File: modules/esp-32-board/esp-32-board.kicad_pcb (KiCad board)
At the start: 2 copper layers, 53.4 x 68.6 mm, 39 parts, among them J1 Conn_01x14_Female, J2 Conn_01x18_Female, J3 Conn_01x06, J4 USB_B_Micro, J5 Barrel_Jack_MountingPin, J6 ESP-PROG-Program, J7 ESP-PROG-Debug, Q1 BCR129S, SW1 SW_Push, SW2 SW_Push, U1 ESP32-WROOM-32, U2 NCP1117-3.3, U3 NCP1117ST50T3G, U4 USBLC6-2SC6, U5 FT232RL

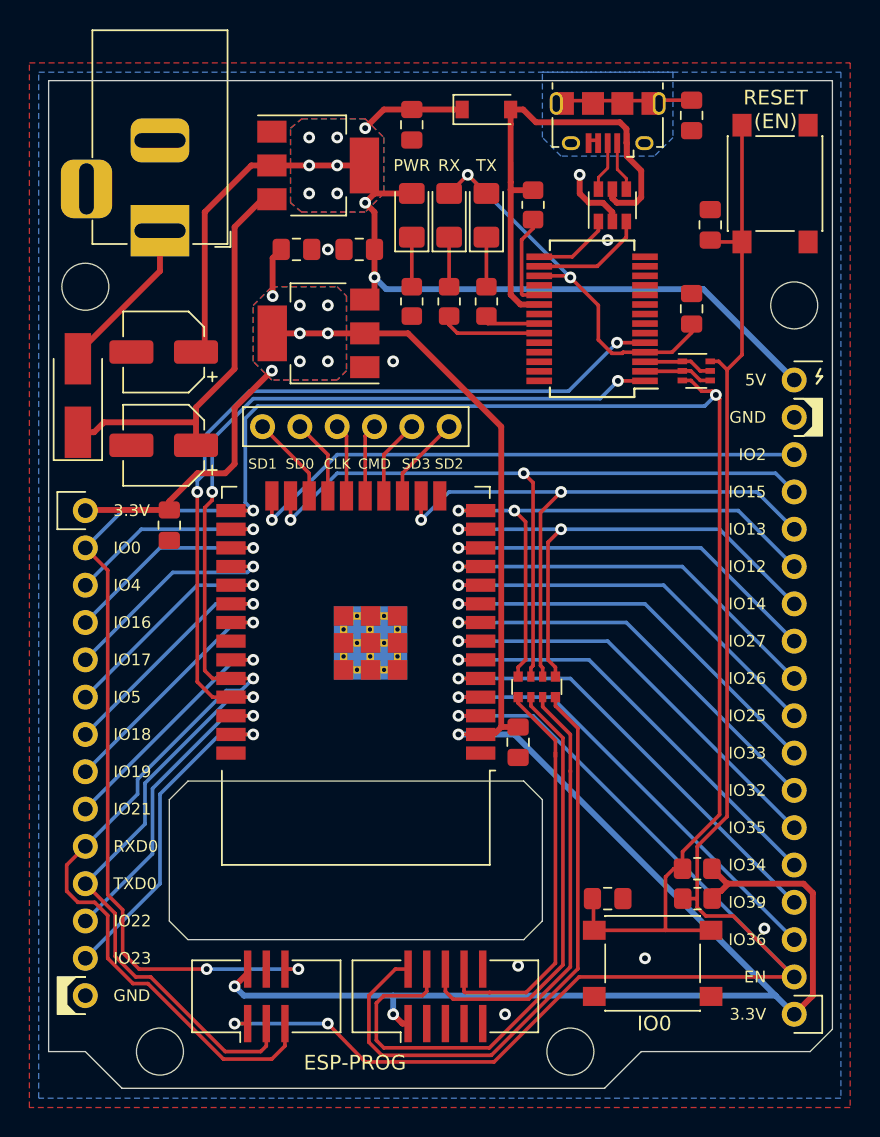
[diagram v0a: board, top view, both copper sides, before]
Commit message: Documentational changes
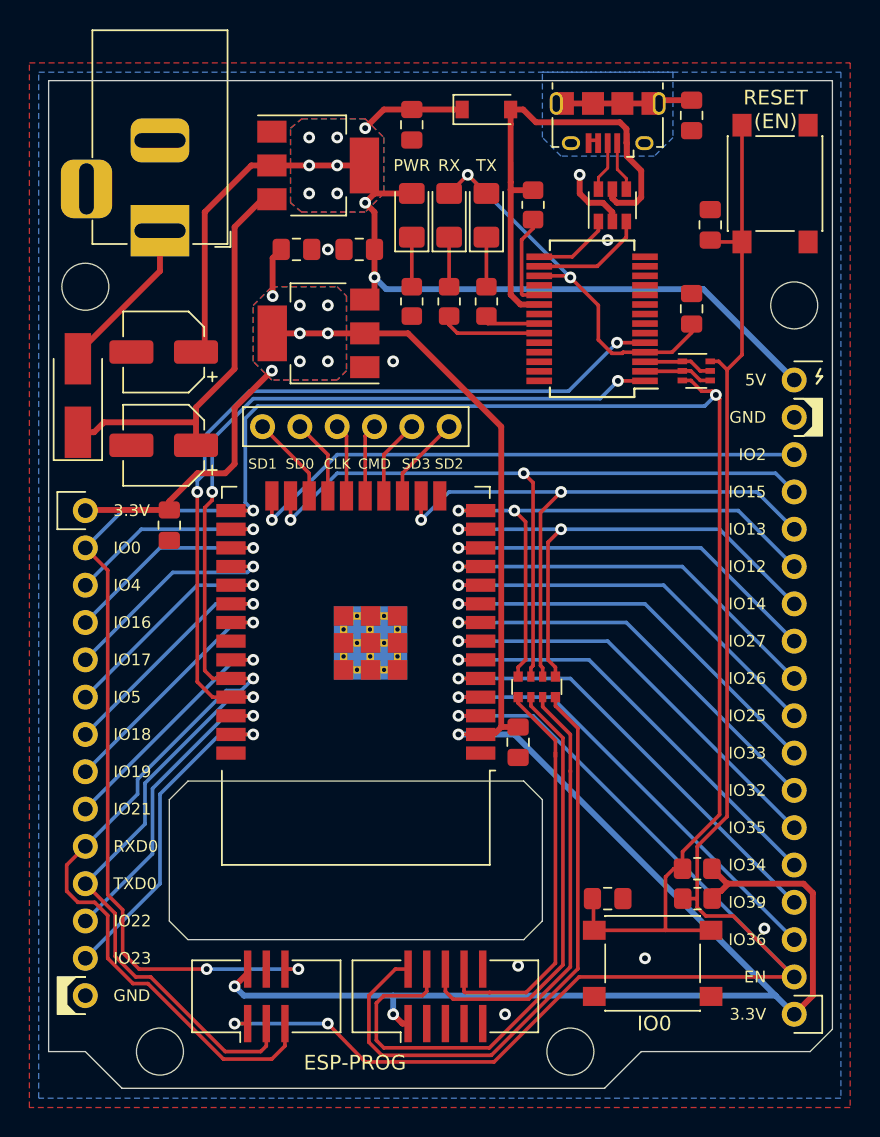
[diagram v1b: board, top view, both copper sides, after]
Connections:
- net Net-(C10-Pad1) renamed /USB/USB_SHIELD
- net Net-(D1-Pad1) renamed /Power/PWR_LED_CATHODE
- net Net-(D2-Pad2) renamed /Power/DC_INPUT
- net Net-(D4-Pad1) renamed /USB/~TXDLED'
- net Net-(D5-Pad1) renamed /USB/~RXDLED'
- net Net-(J4-Pad2) renamed /USB/USB_DN'
- net Net-(J4-Pad3) renamed /USB/USB_DP'
- net Net-(J7-Pad2) renamed /TMS'
- net Net-(J7-Pad4) renamed /TCK'
- net Net-(J7-Pad6) renamed /TDO'
- net Net-(J7-Pad8) renamed /TDI'
- net Net-(R2-Pad1) renamed /USB/USB_RESET
- net VDC renamed /Power/VDC
